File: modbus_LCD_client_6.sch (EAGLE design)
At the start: 32 parts, among them IC4 7805T_H, IC5 ATMEGA328P-PU, J1 9-12V DC CP, Q1 8MHz, Q2 BSS138, Q3 BSS138, U3 BMP180, X1 ISP6IDC

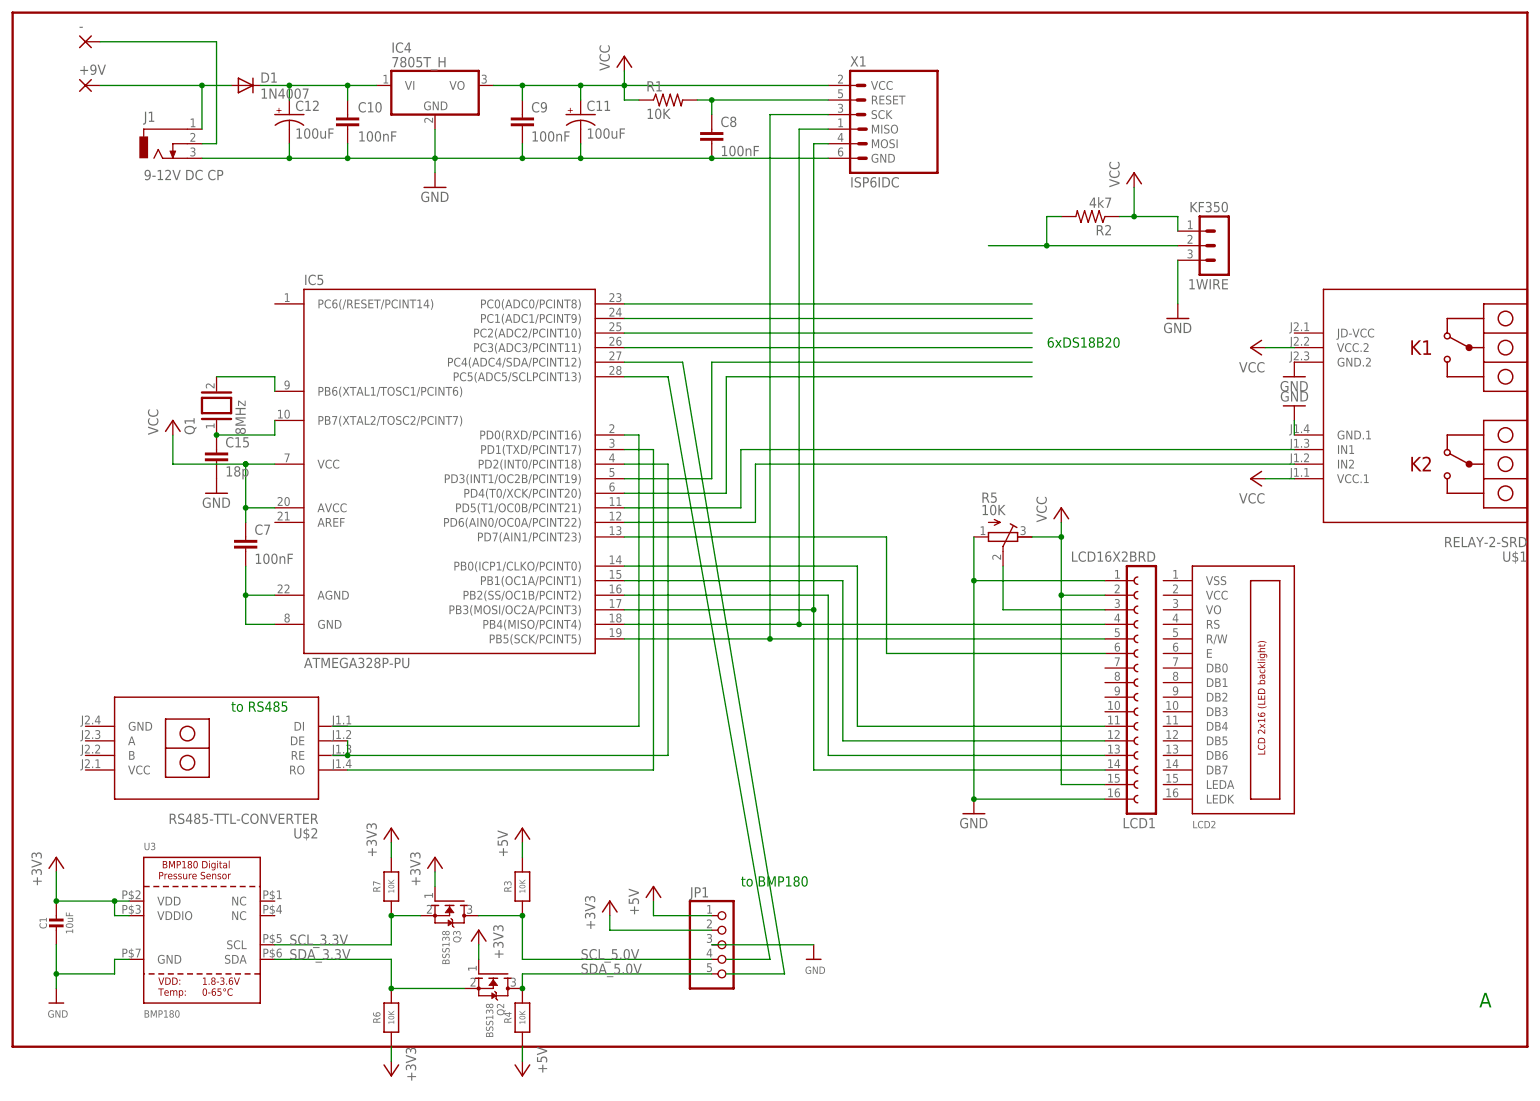
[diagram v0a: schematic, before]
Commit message: Add files via upload
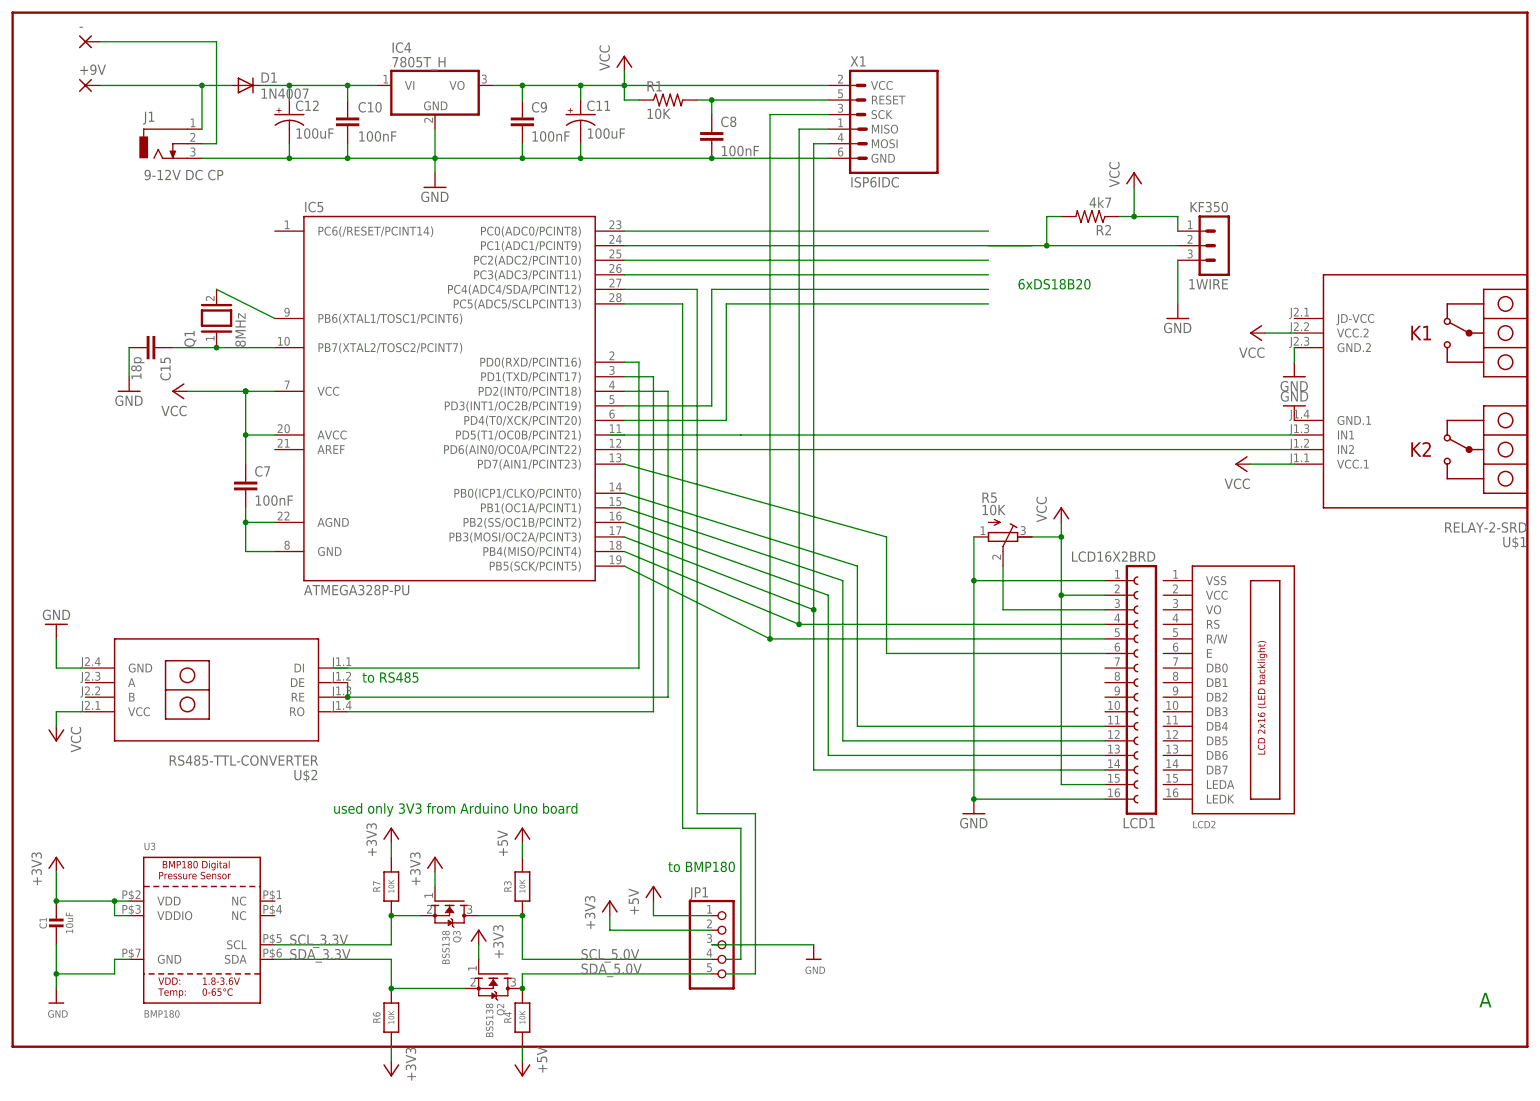
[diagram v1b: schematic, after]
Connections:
- net GND: now also U$2.GND
- net VCC: now also U$2.VCC
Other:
- note added: "used only 3V3 from Arduino Uno board"
- moved on the sheet: C15, C7, IC5, Q1, U$1, U$2
